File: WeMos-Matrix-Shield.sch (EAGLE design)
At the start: 10 parts, among them CN1 1X4-BIG, J2 POWER_JACKPTH, X1 SPTAF_25.0MM

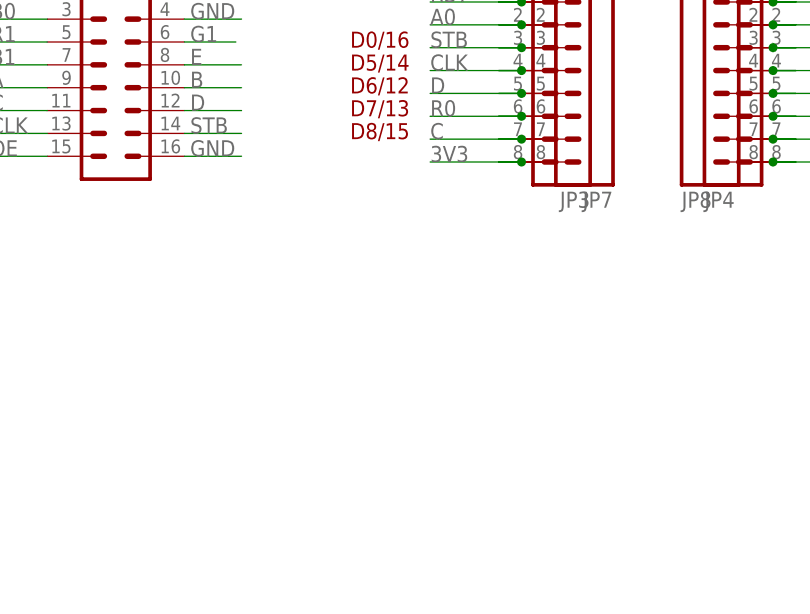
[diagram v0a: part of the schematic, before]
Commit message: Update to V1.2
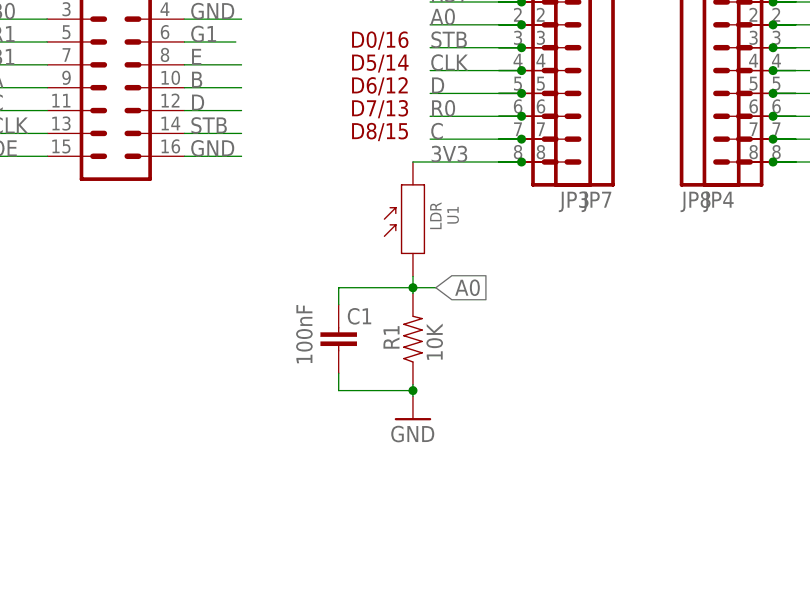
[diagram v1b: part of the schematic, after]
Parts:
- added C1: 100nF, _c2h:CAPPTH2
- added R1: 10K, _c2h:RESISTORPTH-1/6W
- added U1: LDR, Seeed-Sensor:PHOTORESISTOR-5528-10K(2P-5.0X4.2MM)
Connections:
- net 3V3: now also U1.P$2
- net A0: now also C1.1, R1.2, U1.P$1
- net GND: now also C1.2, R1.1
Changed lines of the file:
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@@
 <part name="NAME" library="SparkFun-Aesthetics" deviceset="FRAME-A4L" device="" value="Value">
 <attribute name="CNAME" value="ESP8266 Wemos Matrix Shield"/>
-<attribute name="CREVISION" value="1.1"/>
+<attribute name="CREVISION" value="1.2"/>
 <attribute name="DESIGNER" value="Charles-Henri Hallard"/>
 </part>
@@
 <part name="GND1" library="supply1" deviceset="GND" device=""/>
 <part name="J3" library="SparkFun-Connectors" deviceset="CONN_04" device="SCREW"/>
+<part name="U1" library="Seeed-Sensor" deviceset="PHOTORESISTOR-5528-10K(2P-5.0X4.2MM)" device="" value="LDR"/>
+<part name="R1" library="_c2h" deviceset="RESISTOR" device="PTH-1/6W" value="10K"/>
+<part name="GND2" library="supply1" deviceset="GND" device=""/>
+<part name="C1" library="_c2h" deviceset="CAP" device="PTH2" value="100nF"/>
 </parts>
 <sheets>
@@
 <instance part="GND1" gate="1" x="134.62" y="121.92"/>
 <instance part="J3" gate="G$1" x="140.97" y="141.605" rot="R180"/>
+<instance part="U1" gate="G$1" x="123.825" y="81.28" smashed="yes" rot="R90">
+<attribute name="VALUE" x="125.73" y="83.185" size="1.27" layer="96" ratio="10" rot="R270"/>
+<attribute name="NAME" x="128.905" y="80.645" size="1.27" layer="95" ratio="10" rot="R90"/>
+</instance>
+<instance part="R1" gate="G$1" x="123.825" y="67.945" smashed="yes" rot="R90">
+<attribute name="NAME" x="122.3264" y="66.675" size="1.778" layer="95" rot="R90"/>
+<attribute name="VALUE" x="127.127" y="65.405" size="1.778" layer="96" rot="R90"/>
+</instance>
+<instance part="GND2" gate="1" x="123.825" y="59.055"/>
+<instance part="C1" gate="G$1" x="115.57" y="66.675" smashed="yes">
+<attribute name="NAME" x="116.459" y="69.596" size="1.778" layer="95"/>
+<attribute name="VALUE" x="112.649" y="65.024" size="1.778" layer="96" rot="R90"/>
+</instance>
 </instances>
 <busses>
@@
 <wire x1="149.86" y1="139.065" x2="135.89" y2="139.065" width="0.1524" layer="91"/>
 </segment>
+<segment>
+<pinref part="R1" gate="G$1" pin="1"/>
+<pinref part="GND2" gate="1" pin="GND"/>
+<wire x1="123.825" y1="61.595" x2="123.825" y2="62.23" width="0.1524" layer="91"/>
+<pinref part="C1" gate="G$1" pin="2"/>
+<wire x1="123.825" y1="62.23" x2="123.825" y2="62.865" width="0.1524" layer="91"/>
+<wire x1="123.825" y1="62.23" x2="115.57" y2="62.23" width="0.1524" layer="91"/>
+<wire x1="115.57" y1="62.23" x2="115.57" y2="64.135" width="0.1524" layer="91"/>
+<junction x="123.825" y="62.23"/>
+</segment>
 </net>
 <net name="3V3" class="0">
 <segment>
 <pinref part="JP3" gate="G$1" pin="8"/>
-<wire x1="135.89" y1="87.63" x2="125.73" y2="87.63" width="0.1524" layer="91"/>
+<wire x1="135.89" y1="87.63" x2="123.825" y2="87.63" width="0.1524" layer="91"/>
 <label x="125.73" y="87.63" size="1.778" layer="95"/>
 <pinref part="JP7" gate="G$1" pin="8"/>
 <junction x="135.89" y="87.63"/>
 <wire x1="135.89" y1="87.63" x2="133.35" y2="87.63" width="0.1524" layer="91"/>
+<pinref part="U1" gate="G$1" pin="P$2"/>
 </segment>
 </net>
@@
 <wire x1="135.89" y1="102.87" x2="133.35" y2="102.87" width="0.1524" layer="91"/>
 </segment>
+<segment>
+<pinref part="U1" gate="G$1" pin="P$1"/>
+<wire x1="123.825" y1="74.93" x2="123.825" y2="73.66" width="0.1524" layer="91"/>
+<pinref part="R1" gate="G$1" pin="2"/>
+<wire x1="123.825" y1="73.66" x2="123.825" y2="73.025" width="0.1524" layer="91"/>
+<wire x1="123.825" y1="73.66" x2="126.365" y2="73.66" width="0.1524" layer="91"/>
+<label x="126.365" y="73.66" size="1.778" layer="95" xref="yes"/>
+<junction x="123.825" y="73.66"/>
+<pinref part="C1" gate="G$1" pin="1"/>
+<wire x1="123.825" y1="73.66" x2="115.57" y2="73.66" width="0.1524" layer="91"/>
+<wire x1="115.57" y1="73.66" x2="115.57" y2="71.755" width="0.1524" layer="91"/>
+</segment>
 </net>
